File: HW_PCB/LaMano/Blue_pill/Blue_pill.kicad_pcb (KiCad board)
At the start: 2 copper layers, 38.6 x 55.1 mm, 28 parts, among them J1 V_Battery, J2 STLINK, J5 MPU6050, J6 NRF24, SW1 SW_DPST_x2, SW2 SW_DPST_x2, U1 STM32F103C8Tx, U2 AMS1117-3.3, X1 Crystal

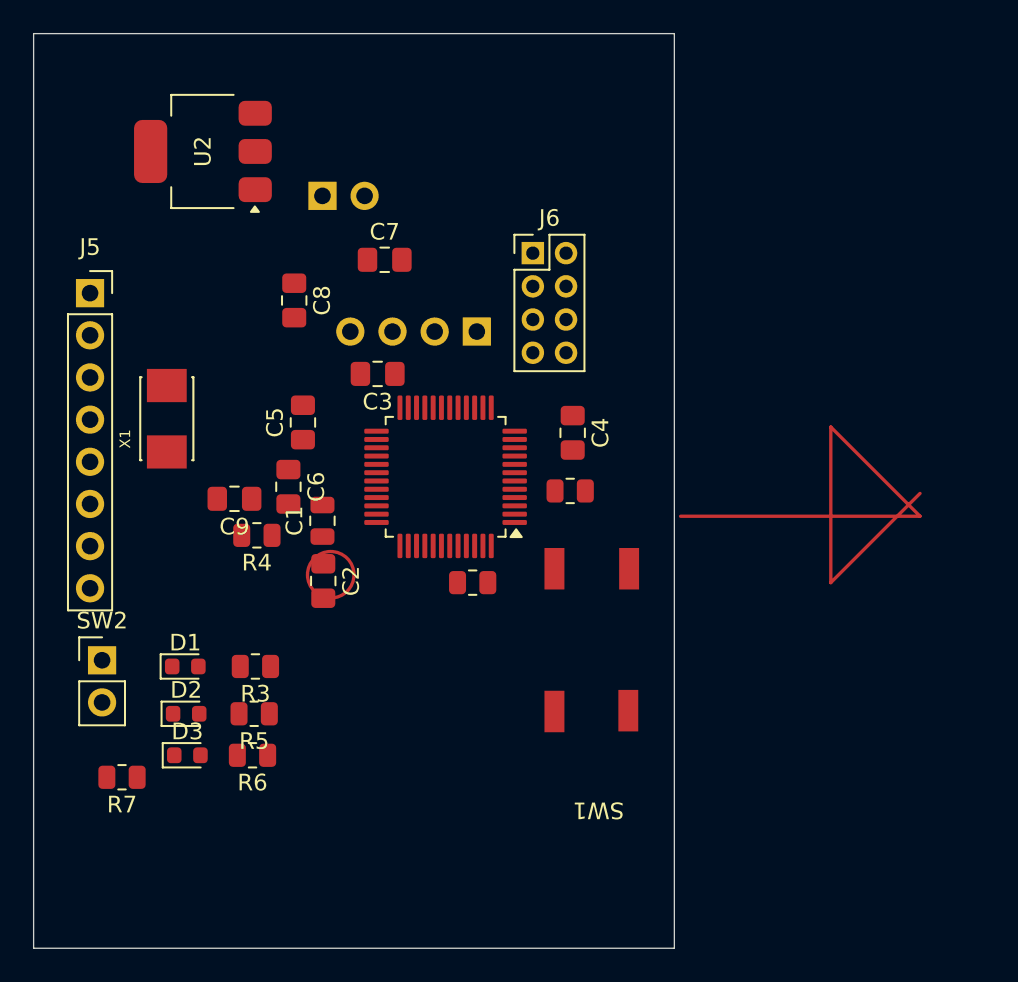
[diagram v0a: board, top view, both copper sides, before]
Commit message: Updated Kicad
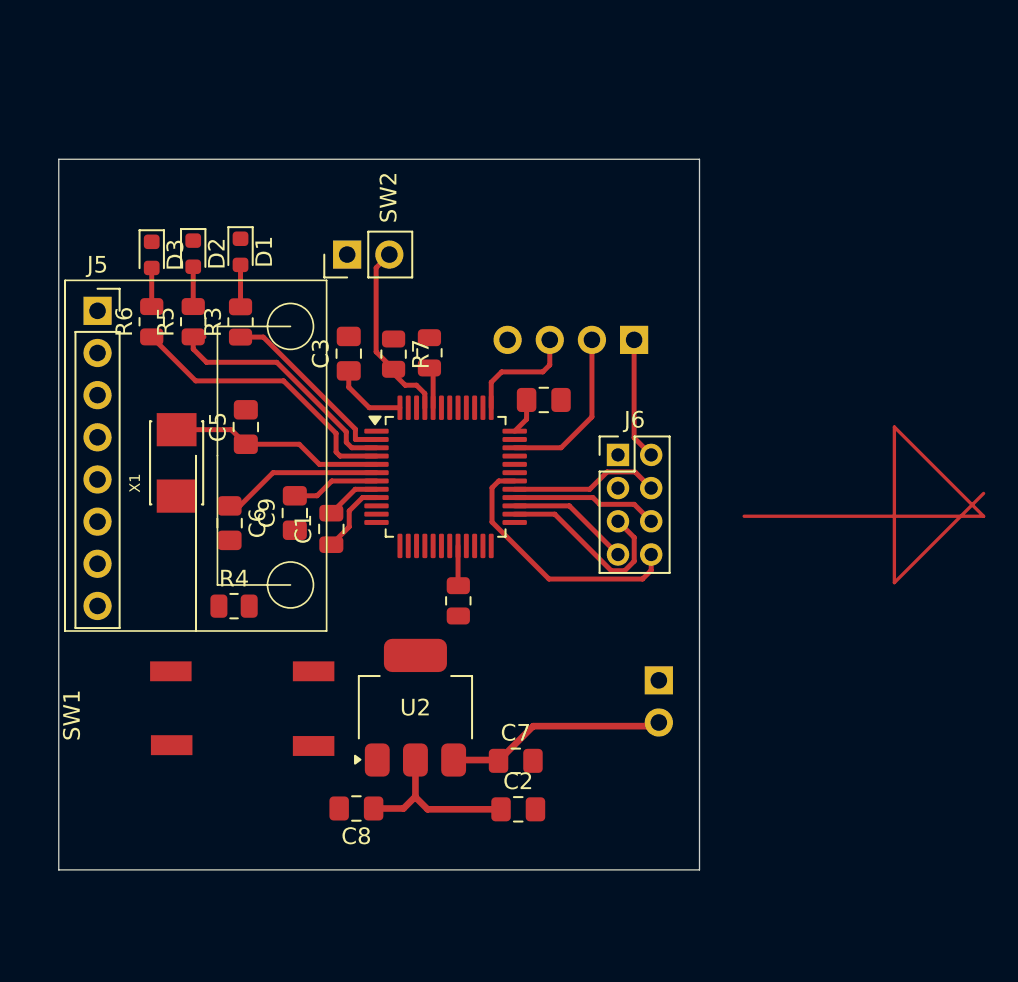
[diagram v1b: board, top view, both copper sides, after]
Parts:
- moved U2 35.9 mm to (57.6, 75.5), turned to 90 degrees
- moved J1 35.5 mm to (72.2, 73.8), turned to 180 degrees
- moved SW1 31.6 mm to (37.4, 75.9), turned to 90 degrees
- moved C7 31.2 mm to (63.6, 78.7)
- moved C8 30.8 mm to (54.0, 81.5), turned to 180 degrees
- moved R7 30.3 mm to (56.3, 54.2), turned to -90 degrees
- moved D3 30.2 mm to (41.7, 48.2), turned to -90 degrees
- moved SW2 28.6 mm to (53.5, 48.2), turned to 90 degrees
- moved D2 27.7 mm to (44.2, 48.1), turned to -90 degrees
- moved R6 26.8 mm to (41.7, 52.2), turned to 90 degrees
- moved D1 25.2 mm to (47.0, 48.0), turned to -90 degrees
- moved R5 23.9 mm to (44.2, 52.2), turned to 90 degrees
- moved R3 20.8 mm to (47.0, 52.2), turned to 90 degrees
- moved C2 18.1 mm to (63.8, 81.6), turned to 0 degrees
- moved R2 14.1 mm to (58.4, 54.1), turned to -90 degrees
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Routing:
- net VCC: track 0.00 -> 29.1 mm
- net GREEN: track 0.00 -> 17.2 mm
- net IRQ: track 0.00 -> 15.8 mm
- net YELLOW: track 0.00 -> 15.3 mm
- net VIN: track 0.00 -> 13.3 mm
- net OSC_IN: track 0.00 -> 12.9 mm
- net SCK: track 0.00 -> 11.7 mm
- net SW_LUZ: track 0.00 -> 11.6 mm
- net RED: track 0.00 -> 11.1 mm
- net OSC_OUT: track 0.00 -> 10.5 mm
- net SWDIO: track 0.00 -> 10.1 mm
- net CSN: track 0.00 -> 9.06 mm
- net MOSI: track 0.00 -> 8.82 mm
- net MISO: track 0.00 -> 7.44 mm
- net SWCLK: track 0.00 -> 7.00 mm
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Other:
- board size 38.6 x 55.1 mm -> 38.6 x 42.8 mm
